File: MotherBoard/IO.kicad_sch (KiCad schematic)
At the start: 12 parts, among them J301 1376357-3, J302 Conn_01x04_Pin, J303 430450200

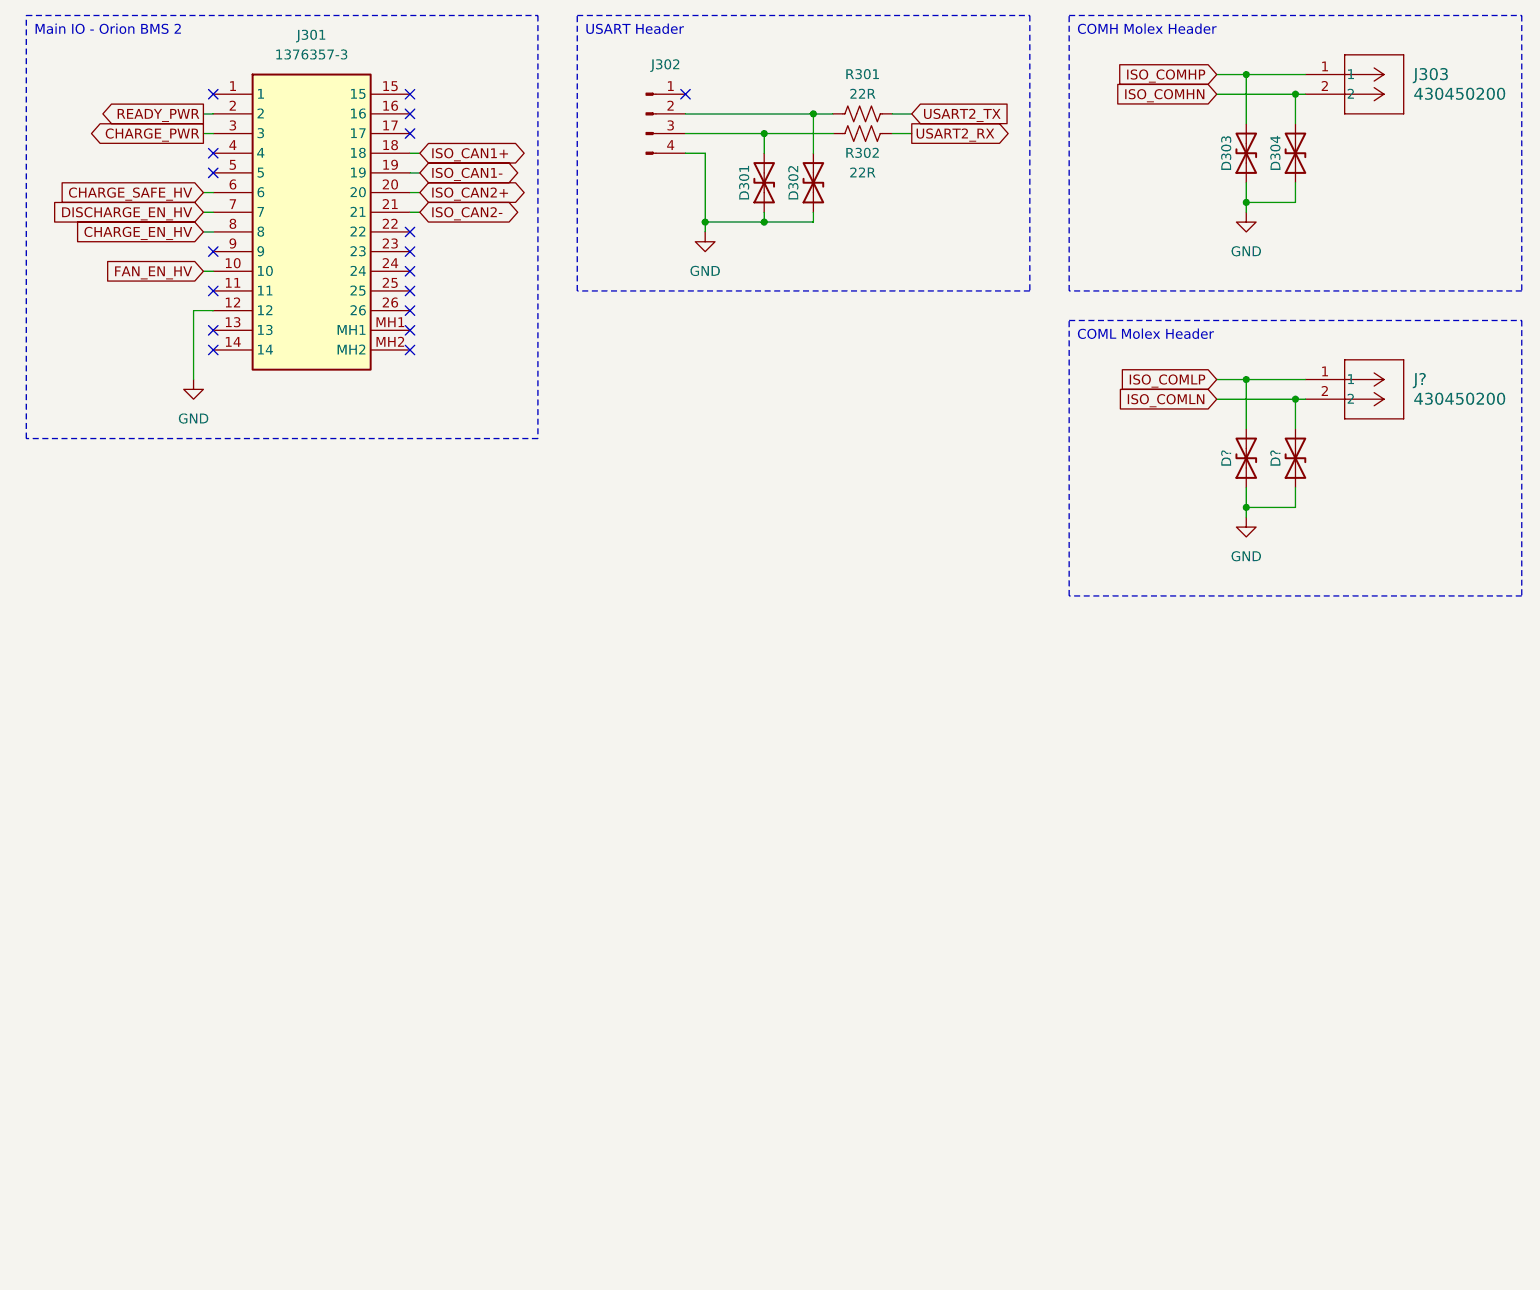
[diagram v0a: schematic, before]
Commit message: Finished motherboard. Need to review BOM
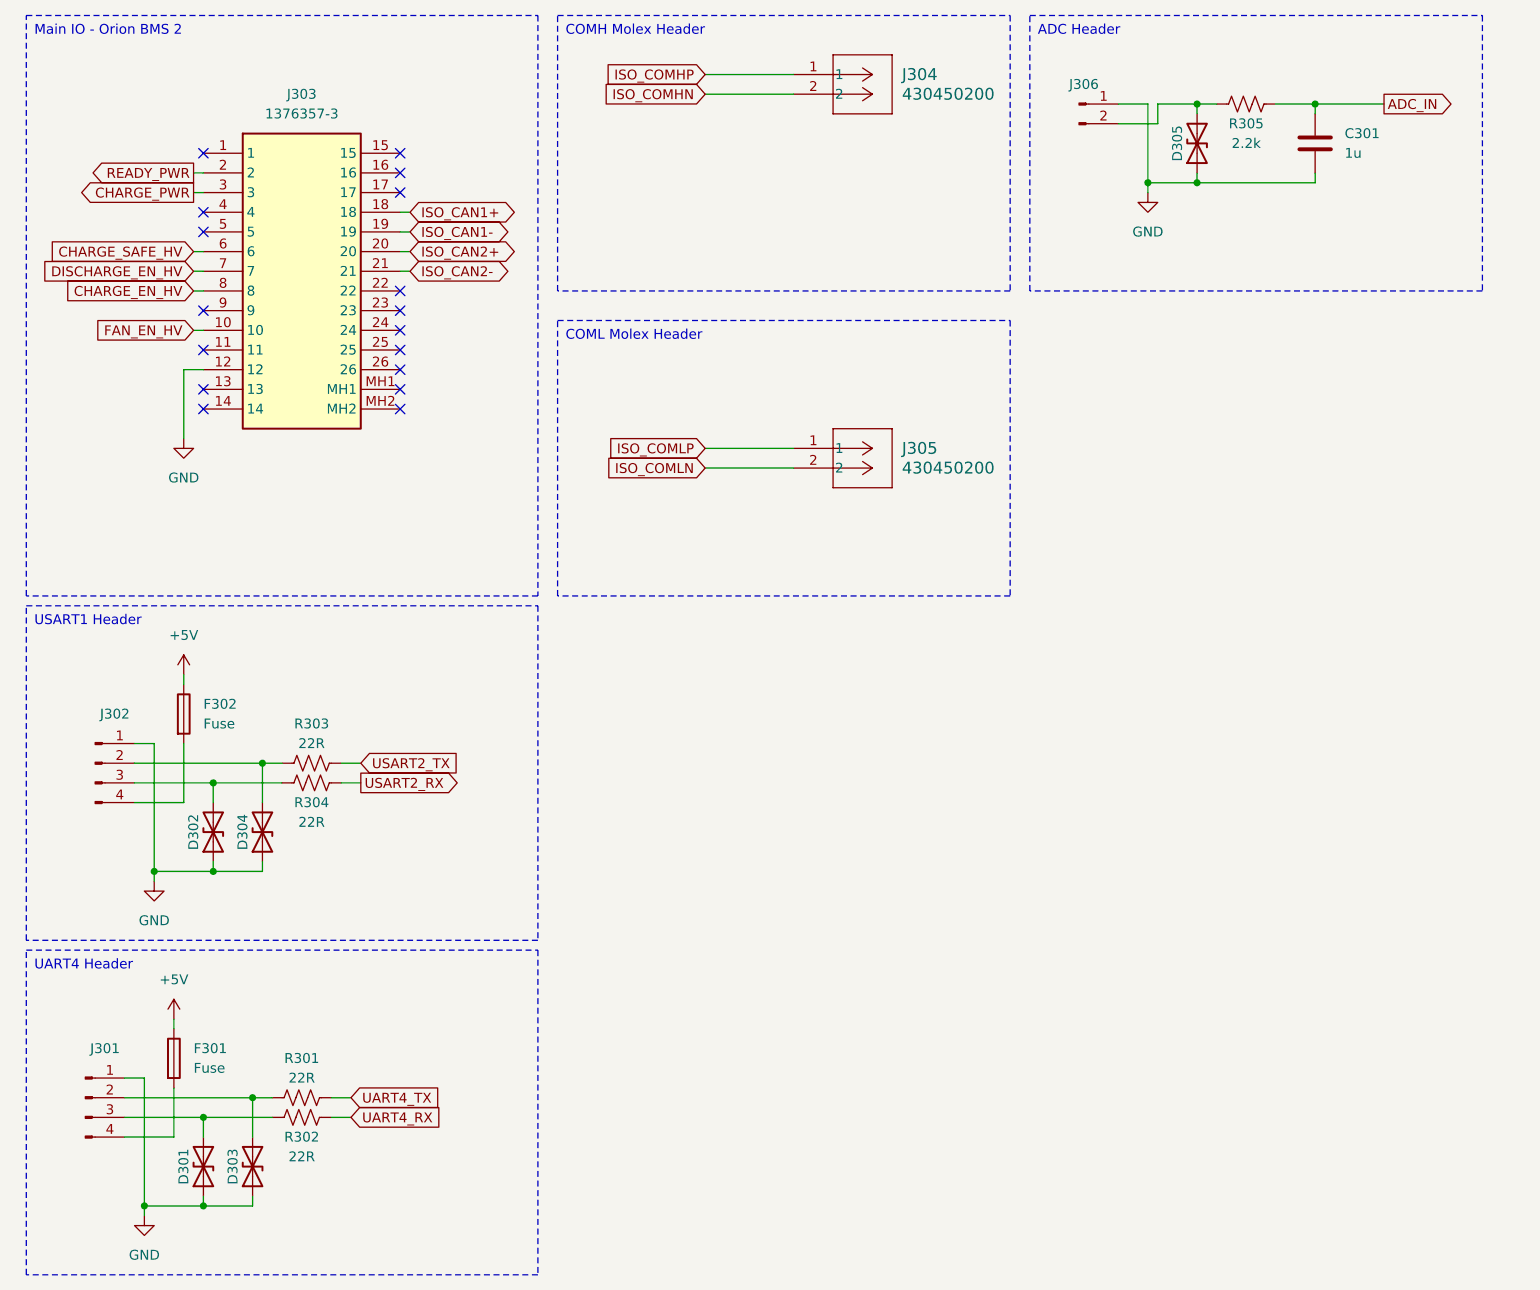
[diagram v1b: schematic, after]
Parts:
- removed D304, D? (x2): D_TVS, Diode_SMD:D_SOD-323, symbol Device:D_TVS
- added C301: 1u, Capacitor_SMD:C_0402_1005Metric, symbol Device:C
- added D301, D305: D_TVS, Diode_SMD:D_SOD-323, symbol Device:D_TVS
- added F301, F302: Fuse, Fuse:Fuse_0805_2012Metric, symbol Device:Fuse
- added J301: Conn_01x04_Pin, Connector_PinHeader_2.54mm:PinHeader_1x04_P2.54mm_Vertical, symbol Connector:Conn_01x04_Pin
- added J306: Conn_01x02_Pin, Connector_PinHeader_2.54mm:PinHeader_1x02_P2.54mm_Vertical, symbol Connector:Conn_01x02_Pin
- added R301, R302: 22R, Resistor_SMD:R_1206_3216Metric, symbol Device:R_US
- added R305: 2.2k, Resistor_SMD:R_1206_3216Metric, symbol Device:R_US
- D303: Manufacturer_Part_Number (none) -> PESD3V3L1BA,115
- gave numbers to parts that had none: 1
- renumbered D301 to D302, D302 to D304, J301 to J303, J303 to J304, R301 to R303, R302 to R304
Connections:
- net GND: now also J302.1 (Pin_1), C301.2, D301.1 (A1), D305.1 (A1), J301.1 (Pin_1), J306.1 (Pin_1); no longer J302.4 (Pin_4)
- net ISO_COMHP: no longer D303.2 (A2)
- new net: D301.2 (A2), J301.3 (Pin_3), R302.1
- new net: D303.2 (A2), J301.2 (Pin_2), R301.1
- new net: F301.2, J301.4 (Pin_4)
- new net: D305.2 (A2), J306.2 (Pin_2), R305.1
- new net: F302.2, J302.4 (Pin_4)
- new net +5V: F301.1, F302.1
- new net ADC_IN: C301.1, R305.2
- new net UART4_RX: R302.2
- new net UART4_TX: R301.2
- no-connect marks 18 -> 17
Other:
- moved on the sheet: D302, D304, J302, J303, J304, J305, R303, R304
